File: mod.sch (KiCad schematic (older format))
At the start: 29 parts, among them J1 MICROUSB, P1 CONN_10, Q2 FDD8870, U1 MCP73831

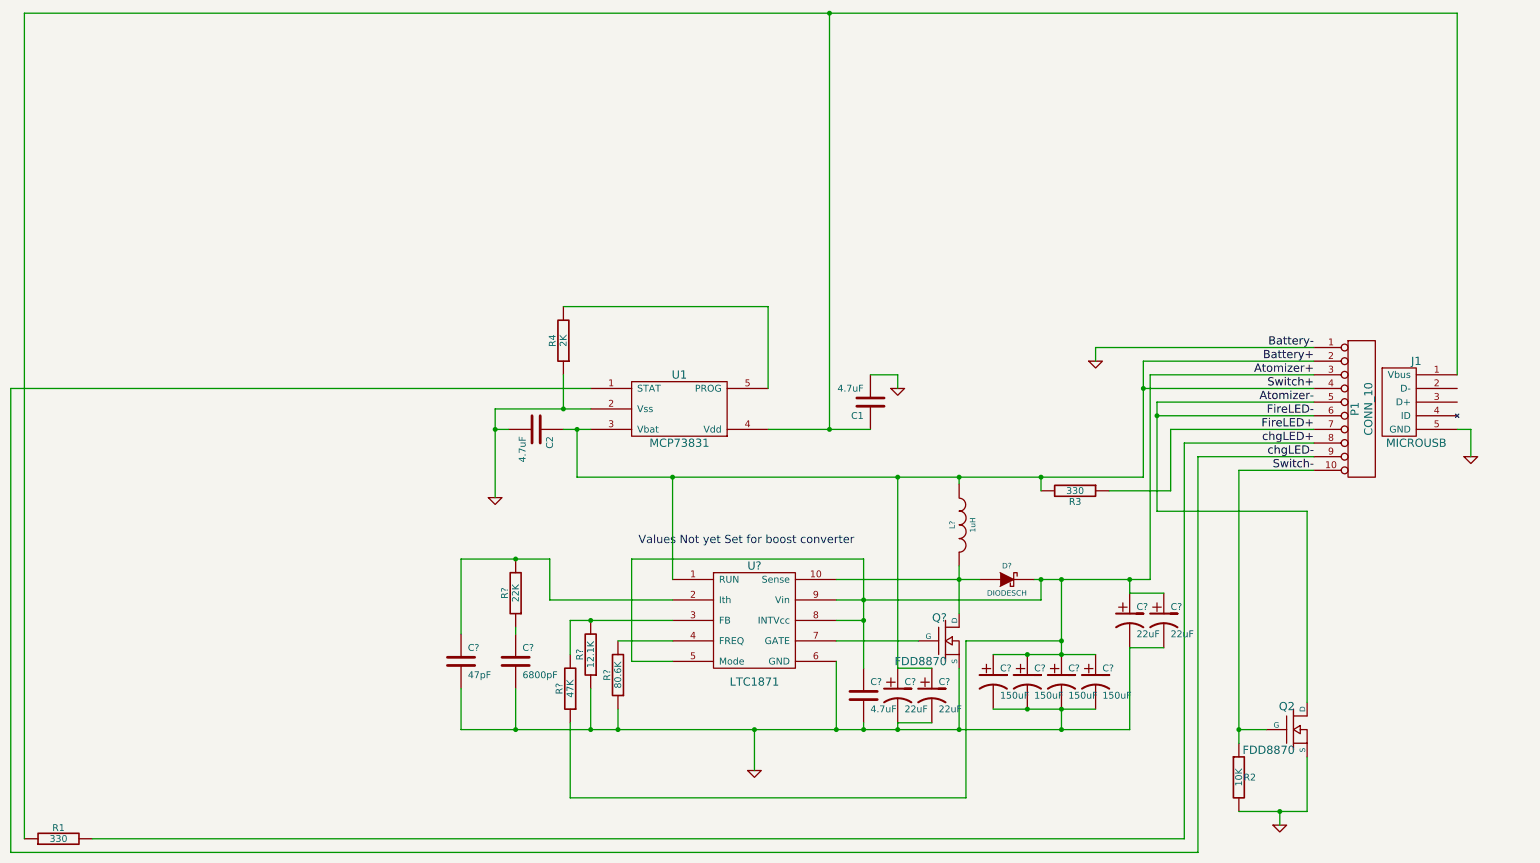
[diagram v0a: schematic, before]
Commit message: progress on booster circuit
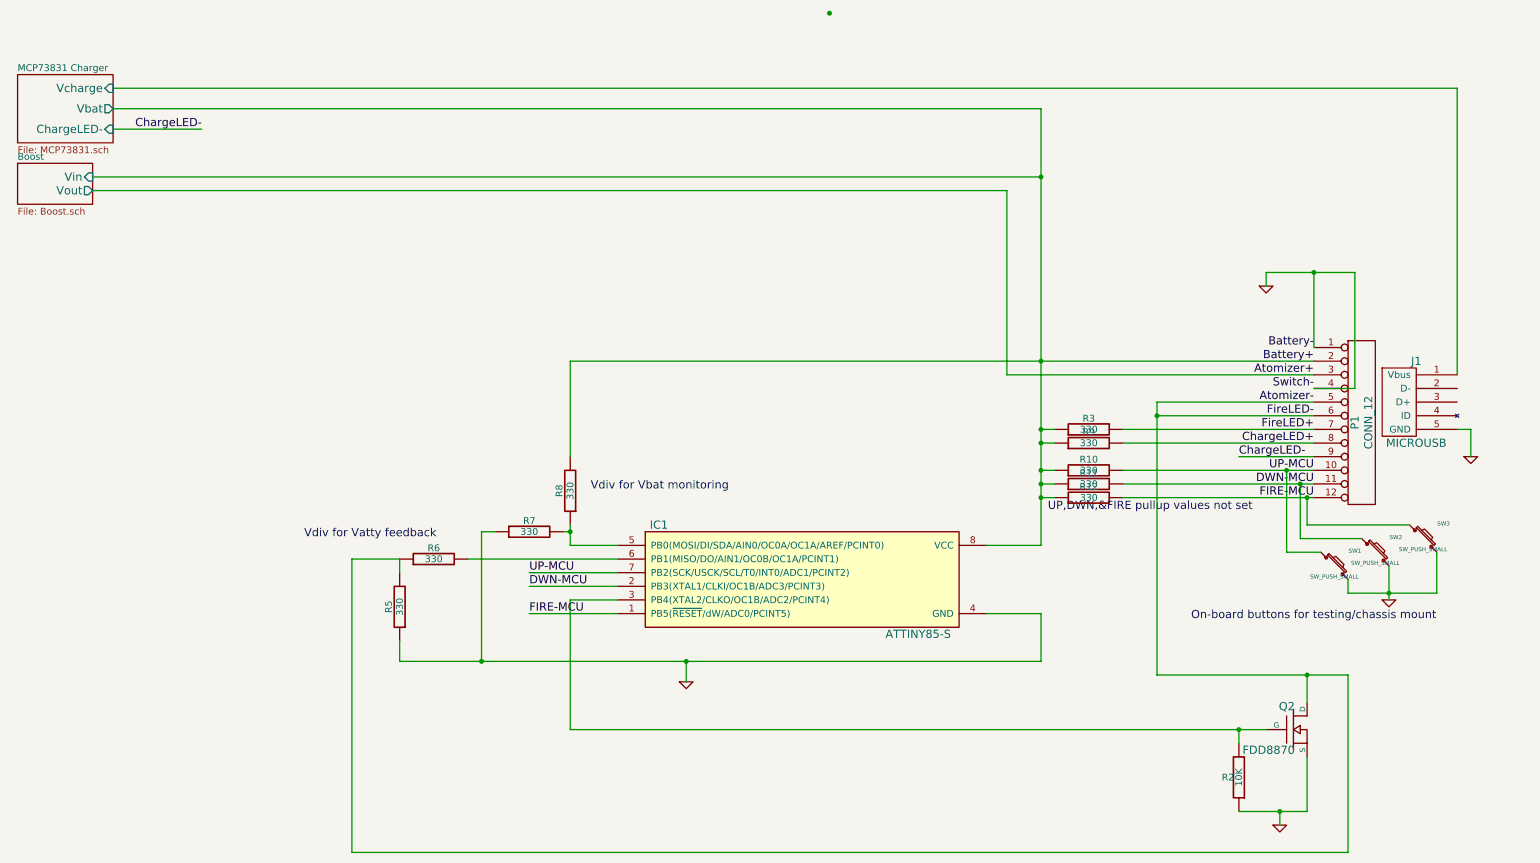
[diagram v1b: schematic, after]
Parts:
- removed C1, C2, C?: 4.7uF, symbol C
- removed C? (x4): 22uF, symbol CP1
- removed C? (x4): 150uF, symbol CP1
- removed C?: 47pF, symbol C
- removed C?: 6800pF, symbol C
- removed D?: DIODESCH, symbol DIODESCH
- removed L?: 1uH, symbol INDUCTOR
- removed P1: CONN_10, symbol CONN_10
- removed Q?: FDD8870, symbol MOSFET_N
- removed R1: 330, symbol R
- removed R4: 2K, symbol R
- removed R?: 22K, symbol R
- removed R?: 47K, symbol R
- removed R?: 12.1K, symbol R
- removed R?: 80.6K, symbol R
- removed U1: MCP73831, ~, symbol MCP73831
- removed U?: LTC1871, ~, symbol LTC1871
- added IC1: ATTINY85-S, SO8-200, symbol ATTINY85-S
- added P1: CONN_12, symbol CONN_12
- added R10, R11, R12, R5, R6, R7, R8, R9: 330, symbol R
- added SW1, SW2, SW3: SW_PUSH_SMALL, symbol SW_PUSH_SMALL
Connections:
- net Atomizer+: now also P1.3 (P3)
- net Atomizer-: now also P1.5 (P5), P1.6 (P6), R5.2, R6.1
- net Battery+: now also R3.1, IC1.8 (VCC), P1.2 (P2), R10.1, R11.1, R12.1, R8.2, R9.1; no longer R3.2
- net FireLED+: now also R3.2, P1.7 (P7); no longer R3.1
- net GND: now also R2.1, IC1.4 (GND), P1.1 (P1), P1.4 (P4), R5.1, R7.1, SW1.2, SW2.2, SW3.2; no longer R2.2
- net MCP73831 Charger/Vcharge: now reaches J1.1 (Vbus)
- net Switch-: no longer names the net of Q2.G
- net Switch-: now also R2.2, IC1.3 (PB4(XTAL2/CLKO/OC1B/ADC2/PCINT4)); no longer R2.1
- new net: IC1.5 (PB0(MOSI/DI/SDA/AIN0/OC0A/OC1A/AREF/PCINT0)), R7.2, R8.1
- new net: IC1.6 (PB1(MISO/DO/AIN1/OC0B/OC1A/PCINT1)), R6.2
- new net ChargeLED+: P1.8 (P8), R9.2
- new net ChargeLED-: P1.9 (P9)
- new net DWN-MCU: IC1.2 (PB3(XTAL1/CLKI/OC1B/ADC3/PCINT3)), P1.11 (P11), R11.2, SW2.1
- new net FIRE-MCU: IC1.1 (PB5(~RESET~/dW/ADC0/PCINT5)), P1.12 (P12), R12.2, SW3.1
- new net UP-MCU: IC1.7 (PB2(SCK/USCK/SCL/T0/INT0/ADC1/PCINT2)), P1.10 (P10), R10.2, SW1.1
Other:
- note added: "On-board buttons for testing/chassis mount"
- note added: "UP,DWN,&FIRE pullup values not set"
- note added: "Vdiv for Vatty feedback"
- note added: "Vdiv for Vbat monitoring"
- note removed: "Values Not yet Set for boost converter"
- moved on the sheet: R3

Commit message: progress on layout
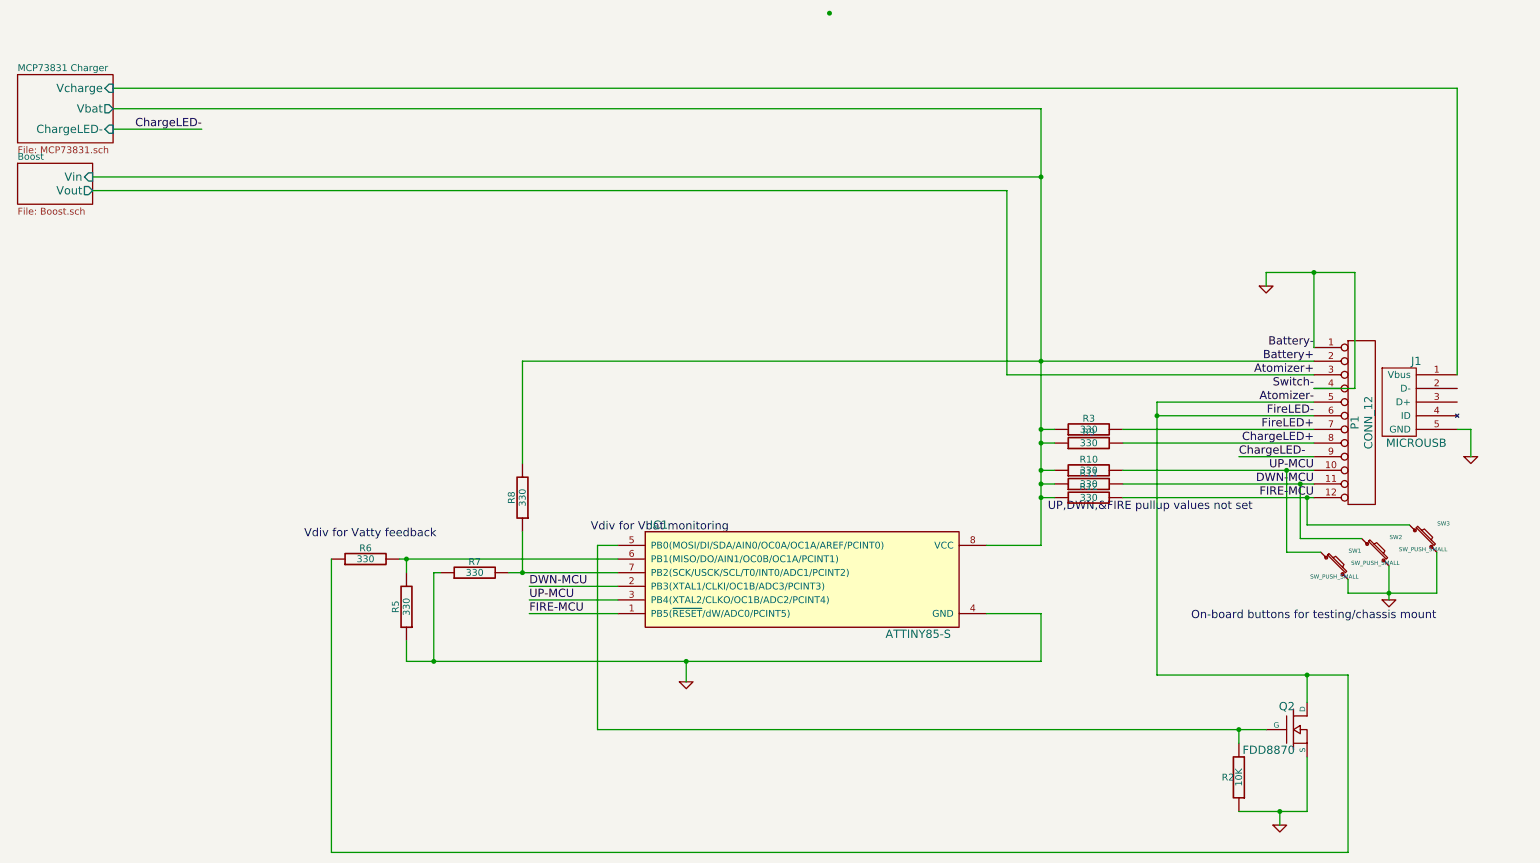
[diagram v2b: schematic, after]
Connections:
- net Atomizer-: no longer R5.2
- net UP-MCU: now also IC1.3 (PB4(XTAL2/CLKO/OC1B/ADC2/PCINT4)); no longer IC1.7 (PB2(SCK/USCK/SCL/T0/INT0/ADC1/PCINT2))
- net at Q2.G, R2.2: now also IC1.5 (PB0(MOSI/DI/SDA/AIN0/OC0A/OC1A/AREF/PCINT0)); no longer IC1.3 (PB4(XTAL2/CLKO/OC1B/ADC2/PCINT4))
- net at R7.2, R8.1: now also IC1.7 (PB2(SCK/USCK/SCL/T0/INT0/ADC1/PCINT2)); no longer IC1.5 (PB0(MOSI/DI/SDA/AIN0/OC0A/OC1A/AREF/PCINT0))
- net at IC1.6 (PB1(MISO/DO/AIN1/OC0B/OC1A/PCINT1)), R6.2: now also R5.2
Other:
- moved on the sheet: R5, R6, R7, R8
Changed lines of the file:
@@
-EESchema Schematic File Version 2  date Fri 29 Mar 2013 12:02:52 PM CDT
+EESchema Schematic File Version 2  date Fri 29 Mar 2013 11:41:29 PM CDT
 LIBS:power
 LIBS:device
@@
 Sheet 1 3
 Title ""
-Date "29 mar 2013"
+Date "30 mar 2013"
 Rev ""
 Comp ""
@@
 Atomizer-
 $Comp
-L GND #PWR3
+L GND #PWR01
 U 1 1 51302ACE
 P 9800 6500
-F 0 "#PWR3" H 9800 6500 30  0001 C CNN
+F 0 "#PWR01" H 9800 6500 30  0001 C CNN
 F 1 "GND" H 9800 6430 30  0001 C CNN
 F 2 "" H 9800 6500 60  0001 C CNN
@@
 Battery+
 $Comp
-L GND #PWR5
+L GND #PWR02
 U 1 1 512C4AF2
 P 11200 3800
-F 0 "#PWR5" H 11200 3800 30  0001 C CNN
+F 0 "#PWR02" H 11200 3800 30  0001 C CNN
 F 1 "GND" H 11200 3730 30  0001 C CNN
 F 2 "" H 11200 3800 60  0001 C CNN
@@
 $EndComp
 $Comp
-L GND #PWR2
+L GND #PWR03
 U 1 1 512AF9E3
 P 9700 2550
-F 0 "#PWR2" H 9700 2550 30  0001 C CNN
+F 0 "#PWR03" H 9700 2550 30  0001 C CNN
 F 1 "GND" H 9700 2480 30  0001 C CNN
 F 2 "" H 9700 2550 60  0001 C CNN
@@
 $EndComp
 $Comp
-L GND #PWR1
+L GND #PWR04
 U 1 1 5155BA90
 P 5450 5450
-F 0 "#PWR1" H 5450 5450 30  0001 C CNN
+F 0 "#PWR04" H 5450 5450 30  0001 C CNN
 F 1 "GND" H 5450 5380 30  0001 C CNN
 F 2 "" H 5450 5450 60  0001 C CNN
@@
 L R R8
 U 1 1 5155BB33
-P 4600 4050
-F 0 "R8" V 4680 4050 50  0000 C CNN
-F 1 "330" V 4600 4050 50  0000 C CNN
-F 2 "" H 4600 4050 60  0001 C CNN
-F 3 "" H 4600 4050 60  0001 C CNN
-	1    4600 4050
+P 4250 4100
+F 0 "R8" V 4330 4100 50  0000 C CNN
+F 1 "330" V 4250 4100 50  0000 C CNN
+F 2 "" H 4250 4100 60  0001 C CNN
+F 3 "" H 4250 4100 60  0001 C CNN
+	1    4250 4100
 	-1   0    0    1
 $EndComp
@@
 L R R7
 U 1 1 5155BB45
-P 4300 4350
-F 0 "R7" V 4380 4350 50  0000 C CNN
-F 1 "330" V 4300 4350 50  0000 C CNN
-F 2 "" H 4300 4350 60  0001 C CNN
-F 3 "" H 4300 4350 60  0001 C CNN
-	1    4300 4350
-	0    -1   -1   0
-$EndComp
-Text Notes 4750 4050 0    60   ~ 0
+P 3900 4650
+F 0 "R7" V 3980 4650 50  0000 C CNN
+F 1 "330" V 3900 4650 50  0000 C CNN
+F 2 "" H 3900 4650 60  0001 C CNN
+F 3 "" H 3900 4650 60  0001 C CNN
+	1    3900 4650
+	0    -1   -1   0
+$EndComp
+Text Notes 4750 4350 0    60   ~ 0
 Vdiv for Vbat monitoring
 $Comp
 L R R6
 U 1 1 5155BC78
-P 3600 4550
-F 0 "R6" V 3680 4550 50  0000 C CNN
-F 1 "330" V 3600 4550 50  0000 C CNN
-F 2 "" H 3600 4550 60  0001 C CNN
-F 3 "" H 3600 4550 60  0001 C CNN
-	1    3600 4550
+P 3100 4550
+F 0 "R6" V 3180 4550 50  0000 C CNN
+F 1 "330" V 3100 4550 50  0000 C CNN
+F 2 "" H 3100 4550 60  0001 C CNN
+F 3 "" H 3100 4550 60  0001 C CNN
+	1    3100 4550
 	0    -1   -1   0
 $EndComp
@@
 L R R5
 U 1 1 5155C2FA
-P 3350 4900
-F 0 "R5" V 3430 4900 50  0000 C CNN
-F 1 "330" V 3350 4900 50  0000 C CNN
-F 2 "" H 3350 4900 60  0001 C CNN
-F 3 "" H 3350 4900 60  0001 C CNN
-	1    3350 4900
+P 3400 4900
+F 0 "R5" V 3480 4900 50  0000 C CNN
+F 1 "330" V 3400 4900 50  0000 C CNN
+F 2 "" H 3400 4900 60  0001 C CNN
+F 3 "" H 3400 4900 60  0001 C CNN
+	1    3400 4900
 	-1   0    0    1
 $EndComp
@@
 	10050 2450 10050 3000
 Wire Wire Line
-	4600 3100 10050 3100
+	4250 3100 8050 3100
+Wire Wire Line
+	8050 3100 10050 3100
 Wire Wire Line
 	11100 3600 11200 3600
@@
 	11200 3600 11200 3800
 Wire Wire Line
-	8900 3400 8900 5400
-Wire Wire Line
-	8900 5400 10300 5400
+	8900 3400 8900 3500
+Wire Wire Line
+	8900 3500 8900 5400
+Wire Wire Line
+	8900 5400 10000 5400
+Wire Wire Line
+	10000 5400 10300 5400
 Wire Wire Line
 	10000 5400 10000 5600
@@
 	10000 6400 10000 6000
 Wire Wire Line
-	9500 6400 10000 6400
+	9500 6400 9800 6400
+Wire Wire Line
+	9800 6400 10000 6400
 Wire Wire Line
 	9800 6400 9800 6500
@@
 Connection ~ 8050 3100
 Wire Wire Line
-	9700 2450 10350 2450
+	9700 2450 10050 2450
+Wire Wire Line
+	10050 2450 10350 2450
 Wire Wire Line
 	9700 2450 9700 2550
@@
 	5450 5300 5450 5450
 Wire Wire Line
-	3350 5300 8050 5300
+	3400 5300 3600 5300
+Wire Wire Line
+	3600 5300 5450 5300
+Wire Wire Line
+	5450 5300 8050 5300
 Connection ~ 5450 5300
 Wire Wire Line
-	4600 3800 4600 3100
-Wire Wire Line
-	3000 6700 10300 6700
+	4250 3850 4250 3100
+Wire Wire Line
+	2850 6700 10300 6700
 Wire Wire Line
 	10300 6700 10300 5400
@@
 	8050 4950 7650 4950
 Wire Wire Line
-	4600 4450 4950 4450
-Wire Wire Line
-	4600 4300 4600 4450
-Wire Wire Line
-	3000 4550 3000 6700
-Wire Wire Line
-	4950 4550 3850 4550
-Wire Wire Line
-	3350 4550 3350 4650
-Wire Wire Line
-	3000 4550 3350 4550
-Wire Wire Line
-	3350 5150 3350 5300
-Wire Wire Line
-	4600 5800 9700 5800
-Wire Wire Line
-	4600 5800 4600 4850
-Wire Wire Line
-	4600 4850 4950 4850
+	4250 4350 4250 4650
+Wire Wire Line
+	2850 4550 2850 6700
+Wire Wire Line
+	3350 4550 3400 4550
+Wire Wire Line
+	3400 4550 4950 4550
+Wire Wire Line
+	3400 5150 3400 5300
+Wire Wire Line
+	4800 5800 9500 5800
+Wire Wire Line
+	9500 5800 9700 5800
 Wire Wire Line
 	9500 5900 9500 5800
@@
 Connection ~ 10050 2450
 Wire Wire Line
-	4550 4350 4600 4350
-Connection ~ 4600 4350
-Wire Wire Line
-	8650 4100 10050 4100
-Wire Wire Line
-	4050 4350 3950 4350
-Wire Wire Line
-	3950 4350 3950 5300
-Connection ~ 3950 5300
+	4150 4650 4250 4650
+Wire Wire Line
+	4250 4650 4950 4650
+Connection ~ 4250 4650
+Wire Wire Line
+	8650 4100 10000 4100
+Wire Wire Line
+	10000 4100 10050 4100
+Wire Wire Line
+	3650 4650 3600 4650
+Wire Wire Line
+	3600 4650 3600 5300
+Connection ~ 3600 5300
 Wire Wire Line
 	8050 4100 8150 4100
@@
 Connection ~ 8050 4100
 Wire Wire Line
-	8650 4000 10050 4000
-Wire Wire Line
-	8650 3900 10050 3900
-Wire Wire Line
-	8050 1250 8050 4450
+	8650 4000 9950 4000
+Wire Wire Line
+	9950 4000 10050 4000
+Wire Wire Line
+	8650 3900 9850 3900
+Wire Wire Line
+	9850 3900 10050 3900
+Wire Wire Line
+	8050 1250 8050 1750
+Wire Wire Line
+	8050 1750 8050 3100
+Wire Wire Line
+	8050 3100 8050 3600
+Wire Wire Line
+	8050 3600 8050 3700
+Wire Wire Line
+	8050 3700 8050 3900
+Wire Wire Line
+	8050 3900 8050 4000
+Wire Wire Line
+	8050 4000 8050 4100
+Wire Wire Line
+	8050 4100 8050 4450
 Wire Wire Line
 	8150 3600 8050 3600
 Connection ~ 8050 3600
 Wire Wire Line
-	4950 4650 4300 4650
+	4950 4850 4300 4850
 Wire Wire Line
 	4950 4750 4300 4750
@@
 	9850 4500 9850 3900
 Connection ~ 9850 3900
-Text Label 4300 4650 0    60   ~ 0
+Text Label 4300 4850 0    60   ~ 0
 UP-MCU
 Text Label 4300 4750 0    60   ~ 0
@@
 $EndComp
 $Comp
-L GND #PWR4
+L GND #PWR05
 U 1 1 5155E12D
 P 10600 4850
-F 0 "#PWR4" H 10600 4850 30  0001 C CNN
+F 0 "#PWR05" H 10600 4850 30  0001 C CNN
 F 1 "GND" H 10600 4780 30  0001 C CNN
 F 2 "" H 10600 4850 60  0001 C CNN
@@
 $EndComp
 Wire Wire Line
-	10600 4600 10600 4850
+	10600 4600 10600 4800
+Wire Wire Line
+	10600 4800 10600 4850
 Wire Wire Line
 	10300 4700 10300 4800
 Wire Wire Line
-	10300 4800 10950 4800
+	10300 4800 10600 4800
+Wire Wire Line
+	10600 4800 10950 4800
 Connection ~ 10600 4800
 Wire Wire Line
@@
 Text Label 1900 1400 2    60   ~ 0
 ChargeLED-
+Wire Wire Line
+	3400 4650 3400 4550
+Connection ~ 3400 4550
+Wire Wire Line
+	4800 5800 4800 4450
+Wire Wire Line
+	4800 4450 4950 4450
 $EndSCHEMATC
